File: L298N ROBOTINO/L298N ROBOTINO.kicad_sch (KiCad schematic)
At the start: 40 parts, among them U2 L298N, U4 ESP32-DevKitC, U5 NRF24L01_Breakout, U6 L298N

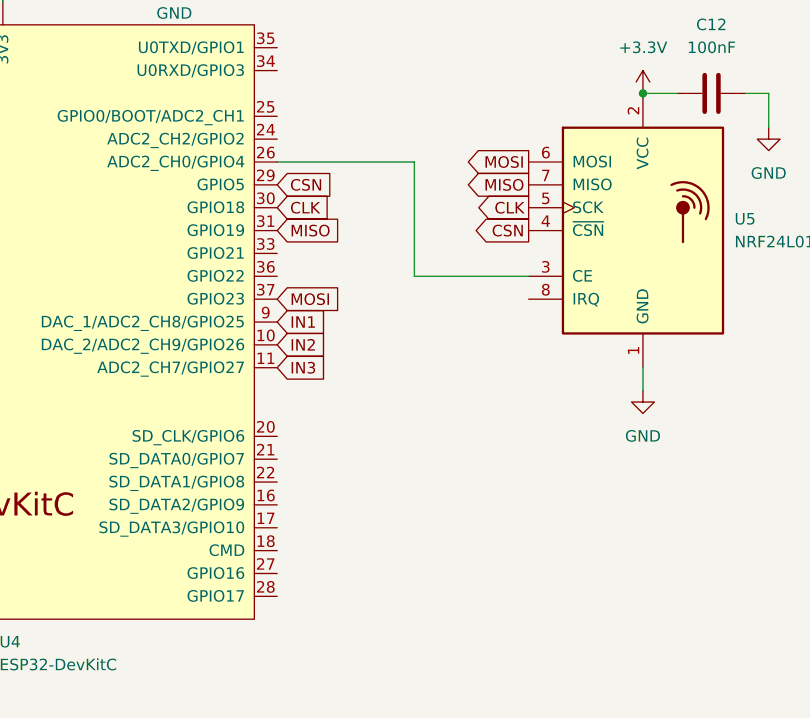
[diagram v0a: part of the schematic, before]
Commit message: New PCB ver 2 Edit
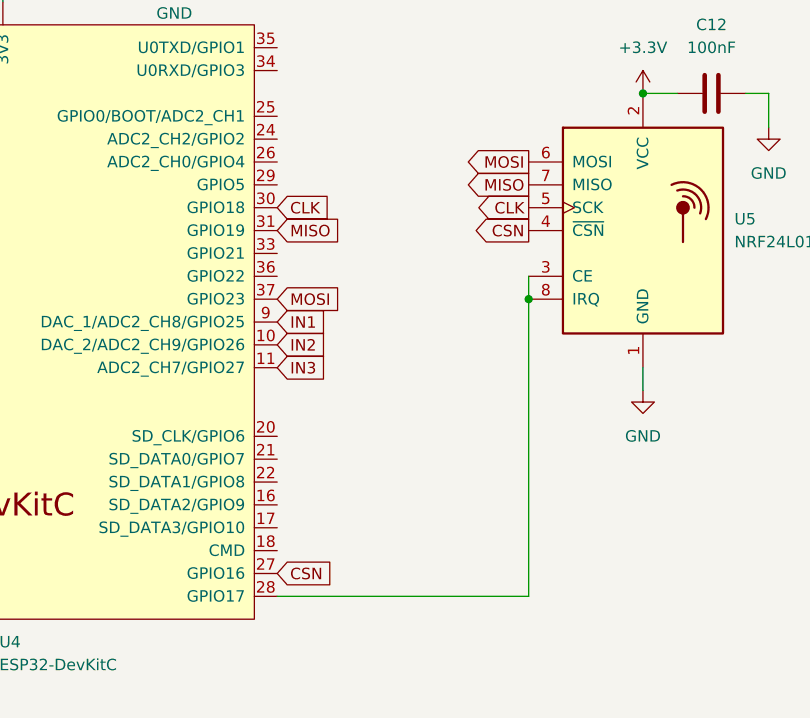
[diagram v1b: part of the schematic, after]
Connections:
- net CSN: now also U4.27 (GPIO16); no longer U4.29 (GPIO5)
- net at U5.3 (CE): now also U4.28 (GPIO17), U5.8 (IRQ); no longer U4.26 (ADC2_CH0/GPIO4)
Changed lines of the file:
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@@
+	)
+	(junction
+		(at 120.65 119.38)
+		(diameter 0)
+		(color 0 0 0 0)
 	)
 	(junction
@@
 	(wire
 		(pts
-			(xy 107.95 116.84) (xy 120.65 116.84)
-		)
-		(stroke
-			(width 0)
-			(type default)
-		)
-	)
-	(wire
-		(pts
 			(xy 101.6 67.31) (xy 107.95 67.31)
 		)
@@
 	(wire
 		(pts
+			(xy 120.65 116.84) (xy 120.65 119.38)
+		)
+		(stroke
+			(width 0)
+			(type default)
+		)
+	)
+	(wire
+		(pts
 			(xy 62.23 74.93) (xy 68.58 74.93)
 		)
@@
 	(wire
 		(pts
+			(xy 120.65 152.4) (xy 92.71 152.4)
+		)
+		(stroke
+			(width 0)
+			(type default)
+		)
+	)
+	(wire
+		(pts
 			(xy 95.25 67.31) (xy 101.6 67.31)
 		)
@@
 	(wire
 		(pts
-			(xy 92.71 104.14) (xy 107.95 104.14)
-		)
-		(stroke
-			(width 0)
-			(type default)
-		)
-	)
-	(wire
-		(pts
 			(xy 27.94 36.83) (xy 27.94 45.72)
 		)
@@
 	(wire
 		(pts
-			(xy 107.95 104.14) (xy 107.95 116.84)
-		)
-		(stroke
-			(width 0)
-			(type default)
-		)
-	)
-	(wire
-		(pts
 			(xy 209.55 106.68) (xy 209.55 121.92)
 		)
@@
 		(pts
 			(xy 68.58 36.83) (xy 71.12 36.83)
+		)
+		(stroke
+			(width 0)
+			(type default)
+		)
+	)
+	(wire
+		(pts
+			(xy 120.65 119.38) (xy 120.65 152.4)
 		)
 		(stroke
@@
 	(global_label "CSN"
 		(shape input)
-		(at 92.71 106.68 0)
+		(at 92.71 149.86 0)
 		(fields_autoplaced yes)
 		(effects
@@
 		)
 		(property "Intersheetrefs" "${INTERSHEET_REFS}"
-			(at 98.851 106.68 0)
-			(hide yes)
-			(show_name no)
+			(at 98.851 149.86 0)
+			(hide yes)
+			(show_name no)
